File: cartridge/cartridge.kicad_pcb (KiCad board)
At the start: 2 copper layers, 63.7 x 92 mm, 31 parts, among them J1 J1B1211CCD, SW1 DS01-254-S-02BE, SW2 CL-SB-13B-01T‎, U1 Teensy4.1, U2 SN74CBTLV3126PWR, U3 SST39VF6401B

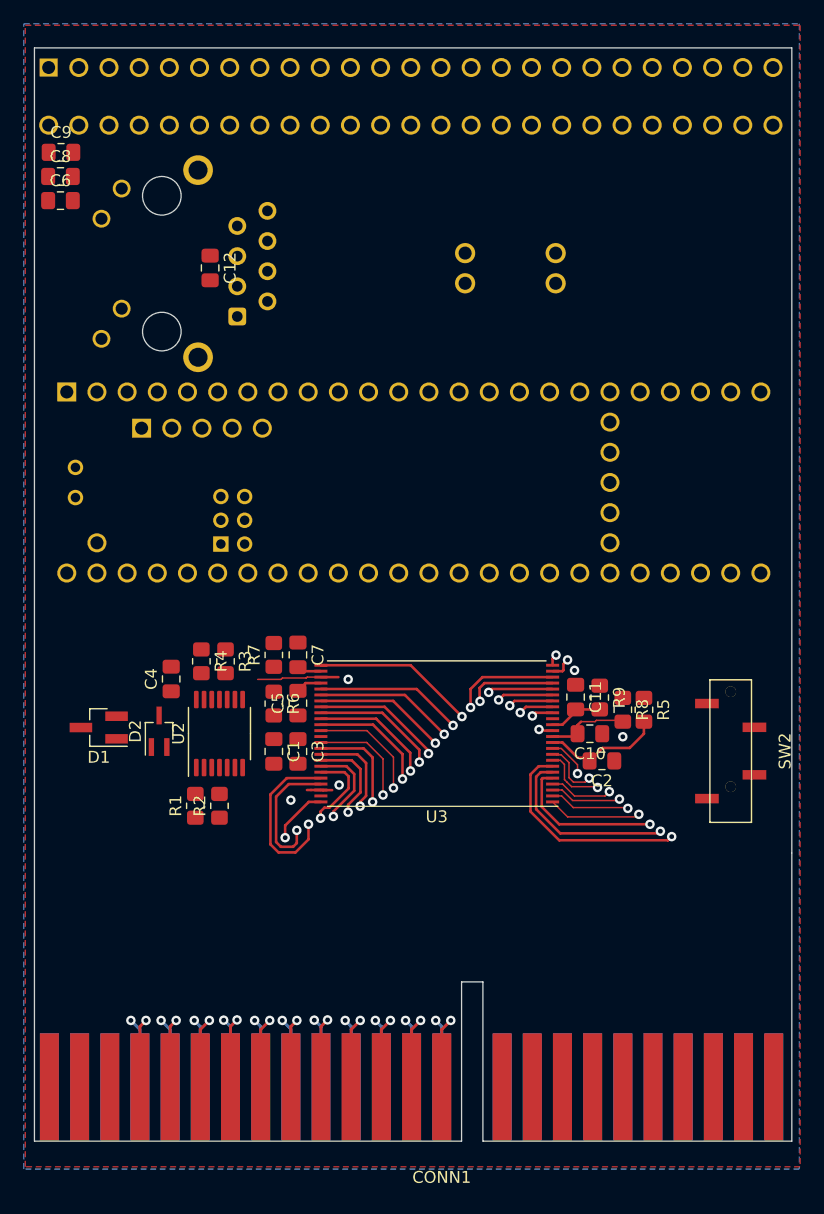
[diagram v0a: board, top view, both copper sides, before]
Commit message: DiscoCart V0.1
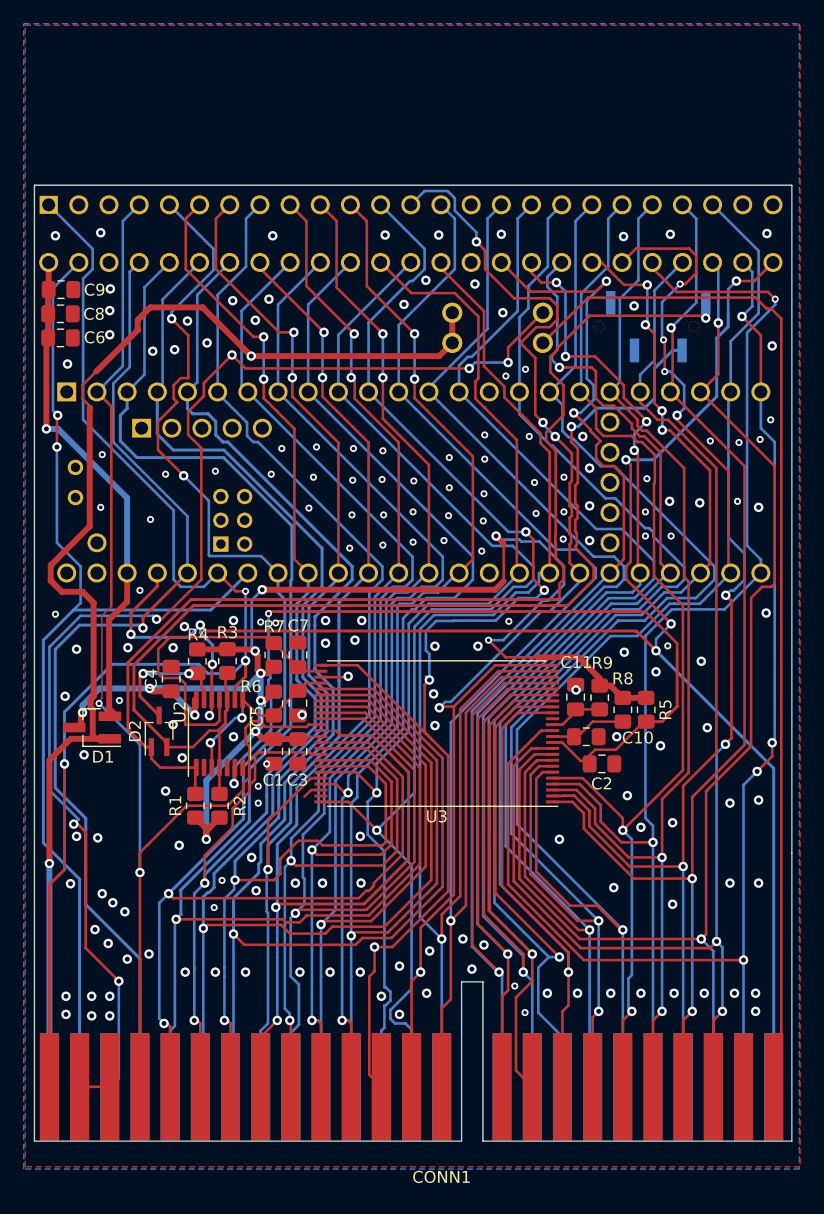
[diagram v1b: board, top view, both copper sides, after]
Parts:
- removed C12: 0.1uF, Capacitor_SMD:C_0805_2012Metric_Pad1.18x1.45mm_HandSolder
- removed J1: J1B1211CCD, Connector_RJ:RJ45_Cetus_J1B1211CCD_Horizontal
- added DISCO-CART: logo, VSmile:logo, F.Cu at (148.6, 115.6)
- SW2: moved to B.Cu
- moved SW2 36.2 mm to (171.4, 73.2), turned to 180 degrees
- moved C6 11.6 mm to (121.1, 74.1)
- moved CONN2 11.6 mm to (150.6, 65.5)
- moved C9 11.6 mm to (121.1, 70.1)
- moved C8 11.6 mm to (121.1, 72.1)
- moved SW1 5.13 mm to (157.9, 73.3)
- moved D1 0.57 mm to (123.7, 106.9)
- moved C10 0.39 mm to (165.3, 107.7)
- moved R4 0.34 mm to (132.6, 101.3)
- moved C2 0.25 mm to (166.6, 110.0)
- moved R5 0.19 mm to (170.4, 105.4)
- moved R3 0.17 mm to (135.1, 101.3)
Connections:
- U1 pad 10: /DQ8 -> /A16
- U1 pad 11: /DQ9 -> /A0
- U1 pad 12: /DQ10 -> /A3
- U1 pad 13: /DQ11 -> /A5
- U1 pad 14: /DQ12 -> /A7
- U1 pad 16: /DQ13 -> /A18
- U1 pad 17: /DQ14 -> /A9
- U1 pad 18: /DQ15 -> /A11
- U1 pad 19: /A0 -> /A13
- U1 pad 2: /DQ0 -> /DQ3
- U1 pad 20: /A1 -> /A14
- U1 pad 21: /A2 -> /A15
- U1 pad 22: /A3 -> /A19
- U1 pad 23: /A4 -> /A20
- U1 pad 24: /A5 -> /A21
- U1 pad 25: /A6 -> /A12
- U1 pad 26: /A7 -> /A10
- U1 pad 28: /A9 -> /A17
- U1 pad 29: /A10 -> /A6
- U1 pad 3: /DQ1 -> /DQ2
- U1 pad 30: /A11 -> /A4
- U1 pad 31: /A12 -> /A1
- U1 pad 32: /A13 -> /A2
- U1 pad 33: /A14 -> /DQ14
- U1 pad 35: /A15 -> /DQ15
- U1 pad 36: /A16 -> /DQ13
- U1 pad 37: /A17 -> /DQ12
- U1 pad 38: /A18 -> /DQ7
- U1 pad 39: /A19 -> /DQ6
- U1 pad 4: /DQ2 -> /DQ1
- U1 pad 40: /A20 -> /DQ5
- U1 pad 41: /A21 -> /DQ4
- U1 pad 5: /DQ3 -> /DQ0
- U1 pad 50: Net-(U1-Pad50) -> GND
- U1 pad 51: Net-(U1-Pad51) -> GND
- U1 pad 52: Net-(U1-Pad52) -> GND
- U1 pad 53: Net-(U1-Pad53) -> GND
- U1 pad 54: Net-(U1-Pad54) -> GND
- U1 pad 55: Net-(U1-Pad55) -> GND
- U1 pad 56: Net-(U1-Pad56) -> GND
- U1 pad 57: Net-(U1-Pad57) -> GND
- U1 pad 58: Net-(U1-Pad58) -> GND
- U1 pad 59: Net-(U1-Pad59) -> GND
- U1 pad 6: /DQ4 -> /DQ11
- U1 pad 60: RX+ -> GND
- U1 pad 61: LED -> GND
- U1 pad 62: TX- -> GND
- U1 pad 63: TX+ -> GND
- U1 pad 65: RX- -> GND
- U1 pad 66: Net-(U1-Pad66) -> GND
- U1 pad 67: Net-(U1-Pad67) -> GND
- U1 pad 7: /DQ5 -> /DQ10
- U1 pad 8: /DQ6 -> /DQ9
- U1 pad 9: /DQ7 -> /DQ8
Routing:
- net /ROM0_1: track 0.00 -> 143.2 mm, vias 0 -> 8
- net /VCC: track 0.00 -> 123.4 mm, vias 0 -> 11
- net /A18: track 1.81 -> 120.9 mm
- net /A7: track 3.77 -> 121.6 mm
- net /A5: track 5.50 -> 119.7 mm
- net /A17: track 2.93 -> 115.9 mm, vias 1 -> 2
- net /DQ4: track 14.6 -> 127.5 mm, vias 2 -> 4
- net /A4: track 7.45 -> 119.4 mm, vias 1 -> 3
- net /DQ2: track 16.5 -> 127.4 mm, vias 2 -> 1
- net /DQ1: track 16.9 -> 127.5 mm, vias 2 -> 1
- net /A20: track 3.41 -> 112.7 mm, vias 1 -> 4
- net /A6: track 4.71 -> 113.8 mm, vias 1 -> 5
- net /A21: track 1.18 -> 109.8 mm, vias 1 -> 4
- net /DQ0: track 18.3 -> 126.6 mm, vias 2 -> 1
- net /VDD_EXT: track 0.00 -> 108.2 mm, vias 0 -> 2
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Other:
- board size 63.7 x 92 mm -> 63.7 x 80.5 mm
- board text added: "DUMP"
- board text added: "STEALTH SWITCH"
